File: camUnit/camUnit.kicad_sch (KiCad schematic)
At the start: 16 parts, among them J1 Conn_01x08, Q1 IRLML6344TRPBF, SW1 SW_SPDT

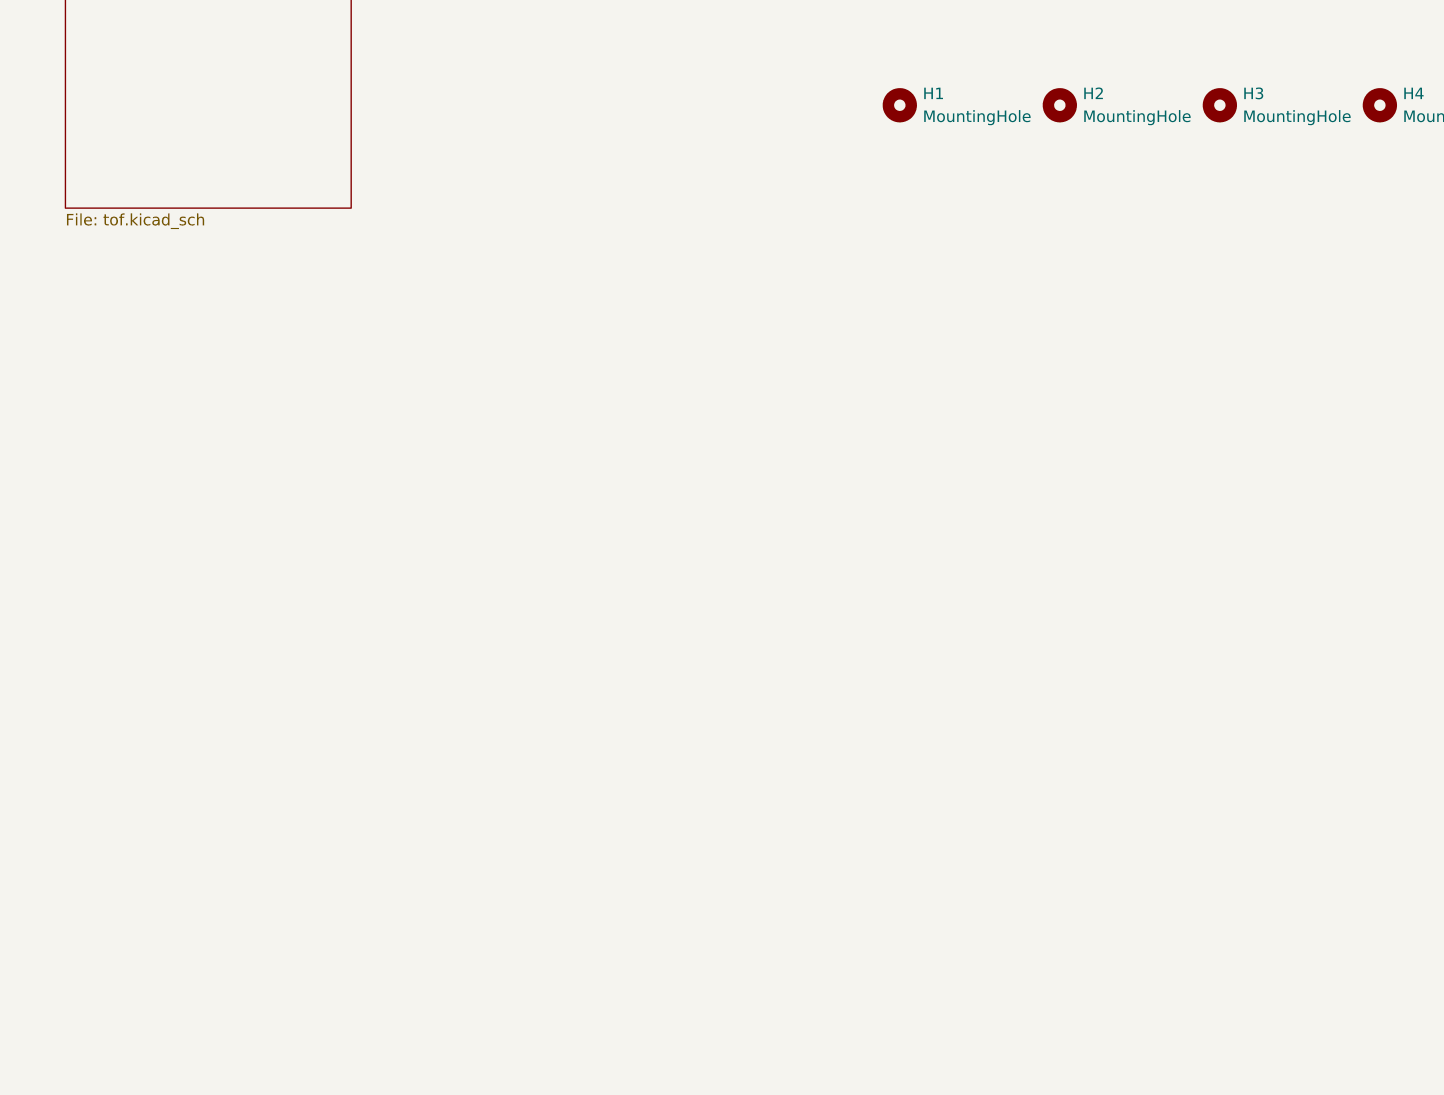
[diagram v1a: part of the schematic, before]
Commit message: Damn u SPI
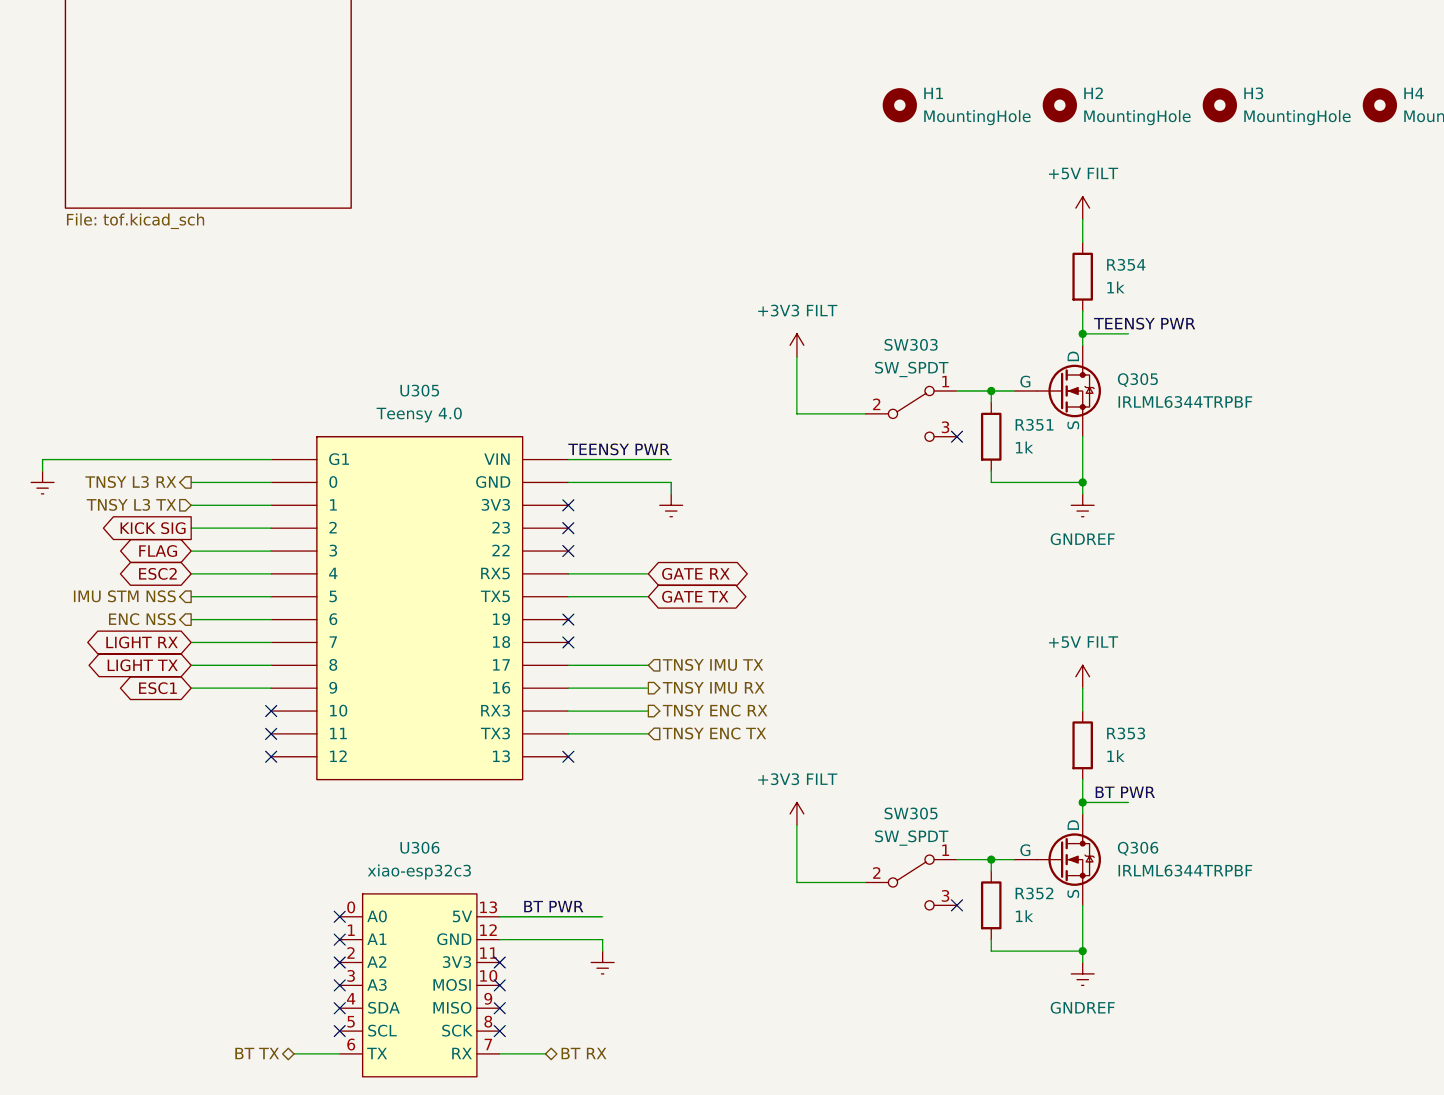
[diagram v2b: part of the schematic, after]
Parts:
- added Q305, Q306: IRLML6344TRPBF, Library:SOT95P237X112-3N, symbol Library:IRLML6344TRPBF
- added R351, R352, R353, R354: 1k, Library:res0603, symbol Device:R
- added SW303, SW305: SW_SPDT, Library:SS12D00G3, symbol Switch:SW_SPDT
- added U305: Teensy 4.0, Library:Teensy 4.0, symbol vincent:Teensy 4.0
- added U306: xiao-esp32c3, Library:xiao-esp32c3, symbol vincent:xiao-esp32c3
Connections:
- net +3V3 FILT: now also SW303.2 (B), SW305.2 (B)
- net +5V FILT: now also R353.1, R354.1
- net GNDREF: now also Q305.2 (S), Q306.2 (S), R351.2, R352.2, U305.G1, U305.G3 (GND), U306.12 (GND)
- new net: Q305.1 (G), R351.1, SW303.1 (A)
- new net: Q306.1 (G), R352.1, SW305.1 (A)
- new net BT PWR: Q306.3 (D), R353.2, U306.13 (5V)
- new net BT RX: U306.7 (RX)
- new net BT TX: U306.6 (TX)
- new net ENC NSS: U305.6
- new net ESC1: U305.9
- new net ESC2: U305.4
- new net FLAG: U305.3
- new net GATE RX: U305.21
- new net GATE TX: U305.20
- new net IMU STM NSS: U305.5
- new net KICK SIG: U305.2
- new net LIGHT RX: U305.7
- new net LIGHT TX: U305.8
- new net TEENSY PWR: Q305.3 (D), R354.2, U305.VIN
- new net TNSY ENC RX: U305.15
- new net TNSY ENC TX: U305.14
- new net TNSY IMU RX: U305.16
- new net TNSY IMU TX: U305.17
- new net TNSY L3 RX: U305.0
- new net TNSY L3 TX: U305.1
- no-connect marks 23 -> 44
